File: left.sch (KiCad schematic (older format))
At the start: 78 parts, among them J1 Speaker, J2 reset, J3 ISP, J9 UTC16-G, P3 WS2812, P4 SJ-43514-SMT, SW1 Socket, SW10 Socket, SW11 Socket, SW12 Socket, SW13 Socket, SW14 Socket, SW15 Socket, SW16 Socket, SW17 Socket, SW18 Socket, SW19 Socket, SW2 Socket, SW20 Socket, SW21 Socket, SW22 Socket, SW23 Socket, SW24 Socket, SW3 Socket, SW4 Socket, SW49 FSMSM, SW5 Socket, SW6 Socket, SW7 Socket, SW8 Socket, SW9 Socket, U1 ATMega32U4, Y1 16MHz

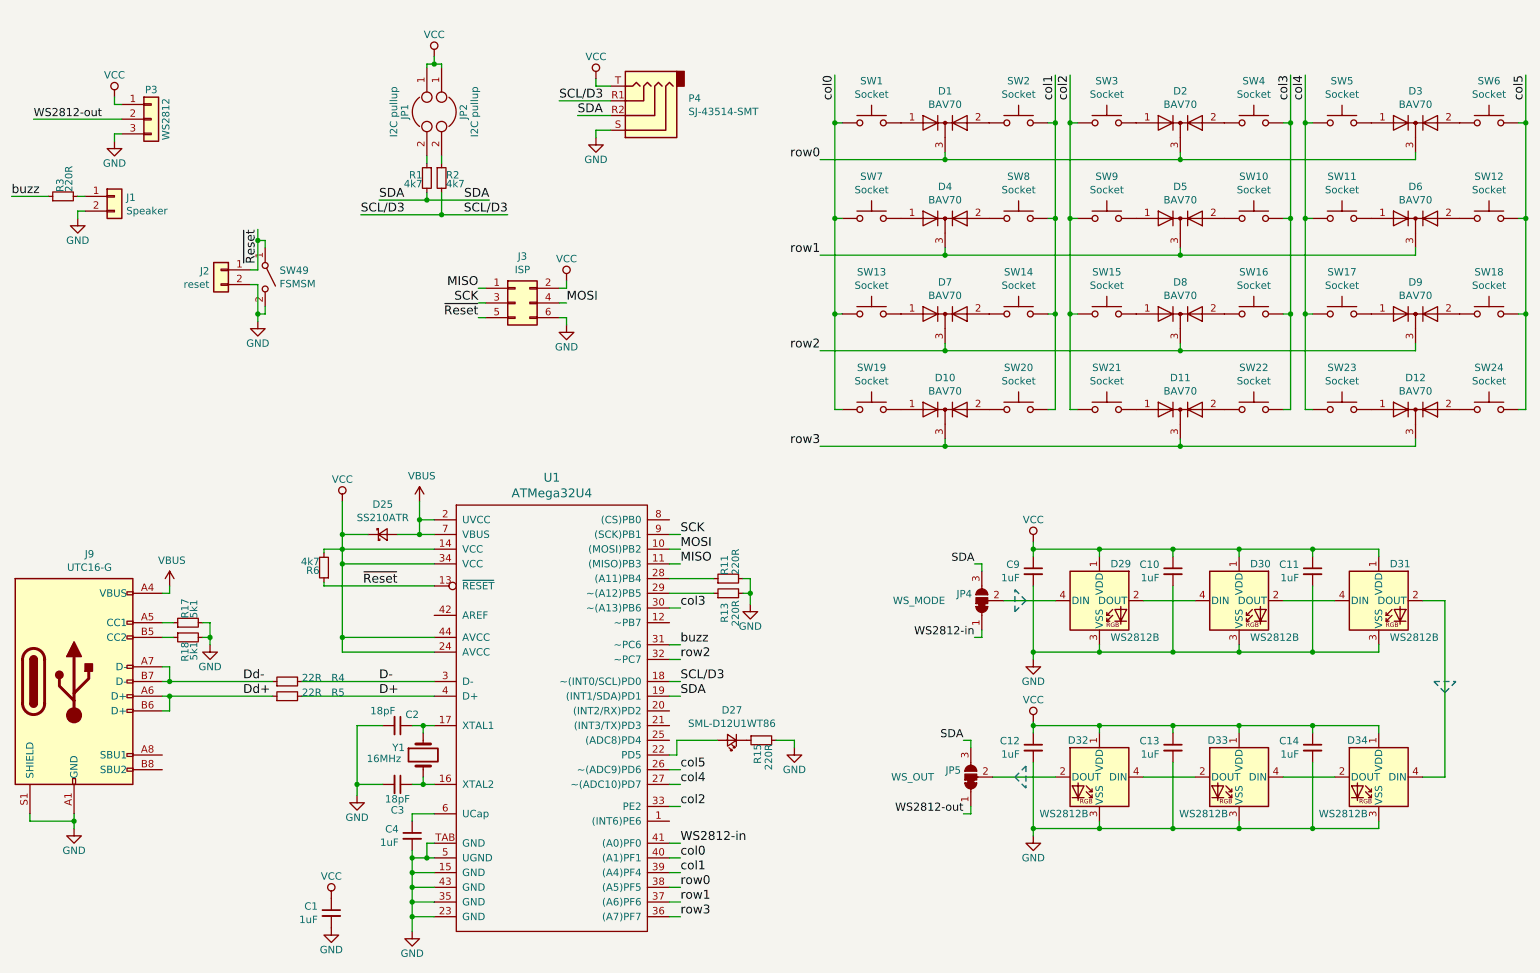
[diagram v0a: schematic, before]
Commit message: Pre-cleanup
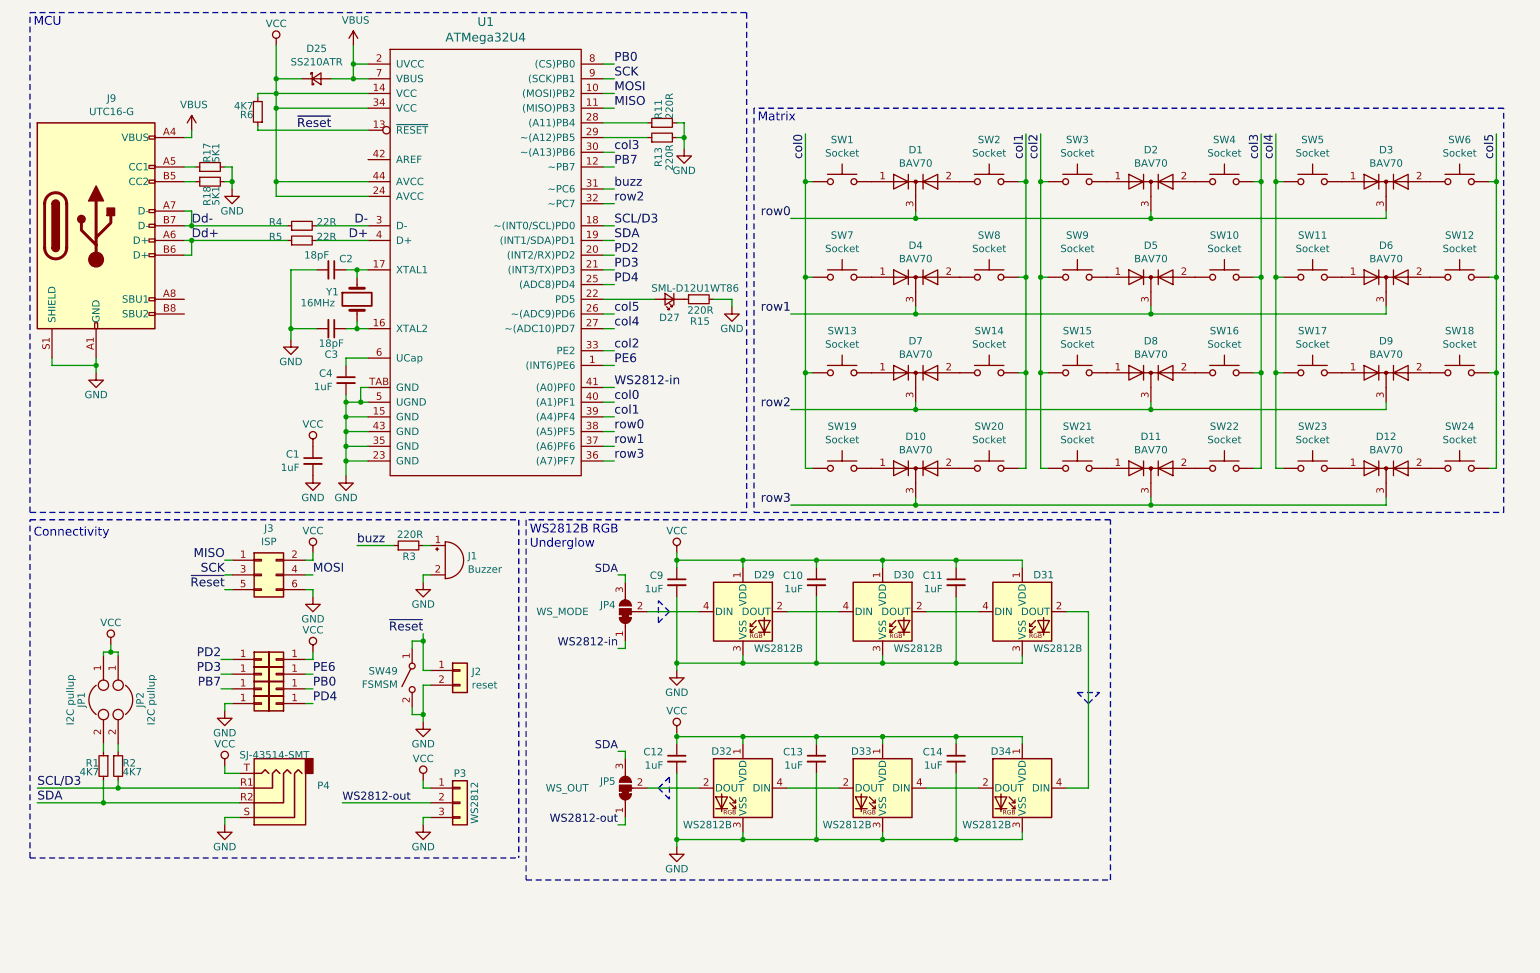
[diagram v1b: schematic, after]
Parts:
- removed J1: Speaker, Buzzers_Beepers:Buzzer_12x9.5RM7.6, symbol vitamins_included-rescue:Conn_01x02-RESCUE-lets_split_panel-lets_split_panel-re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
- added J1: Buzzer, Buzzers_Beepers:Buzzer_12x9.5RM7.6, symbol Device:Buzzer
- added J11, J12, J13, J14, J15, J16, J17, J7: Conn_01x01, TestPoint:TestPoint_Pad_D1.5mm, symbol Connector_Generic:Conn_01x01
- R1, R2, R6: value 4k7 -> 4K7
- R17, R18: value 5k1 -> 5K1
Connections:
- net GND: now also J1.2 (+), J16.1 (Pin_1)
- net VCC: now also J17.1 (Pin_1)
- net at R3.2: now also J1.1 (-)
- net PE6: now reaches U1.1 ((INT6)PE6)
- net PE6: now also J13.1 (Pin_1)
- net PB7: now reaches U1.12 (~~PB7)
- net PB7: now also J14.1 (Pin_1)
- net PD2: now reaches U1.20 ((INT2/RX)PD2)
- net PD2: now also J12.1 (Pin_1)
- net PD3: now reaches U1.21 ((INT3/TX)PD3)
- net PD3: now also J7.1 (Pin_1)
- net PD4: now reaches U1.25 ((ADC8)PD4)
- net PD4: now also J11.1 (Pin_1)
- net PB0: now reaches U1.8 ((CS)PB0)
- net PB0: now also J15.1 (Pin_1)
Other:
- note added: "Connectivity"
- note added: "MCU"
- note added: "Matrix"
- note added: "WS2812B RGB\nUnderglow"
- moved on the sheet: C1, C10, C11, C12, C13, C14, C2, C3, C4, C9, D1, D10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
